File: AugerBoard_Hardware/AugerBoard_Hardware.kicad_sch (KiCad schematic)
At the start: 44 parts, among them J1 RJ45_LED_Shielded, J2 Conn_01x04_MountingPin, Q2 BSS138, Q3 BSS138, SW1 SW_SPDT, SW2 SW_Push, SW3 SW_Push, SW4 SW_Push, U1 Teensy4.1_DEV-16771, U2 OKI-78SR-5_1.5-W36H-C

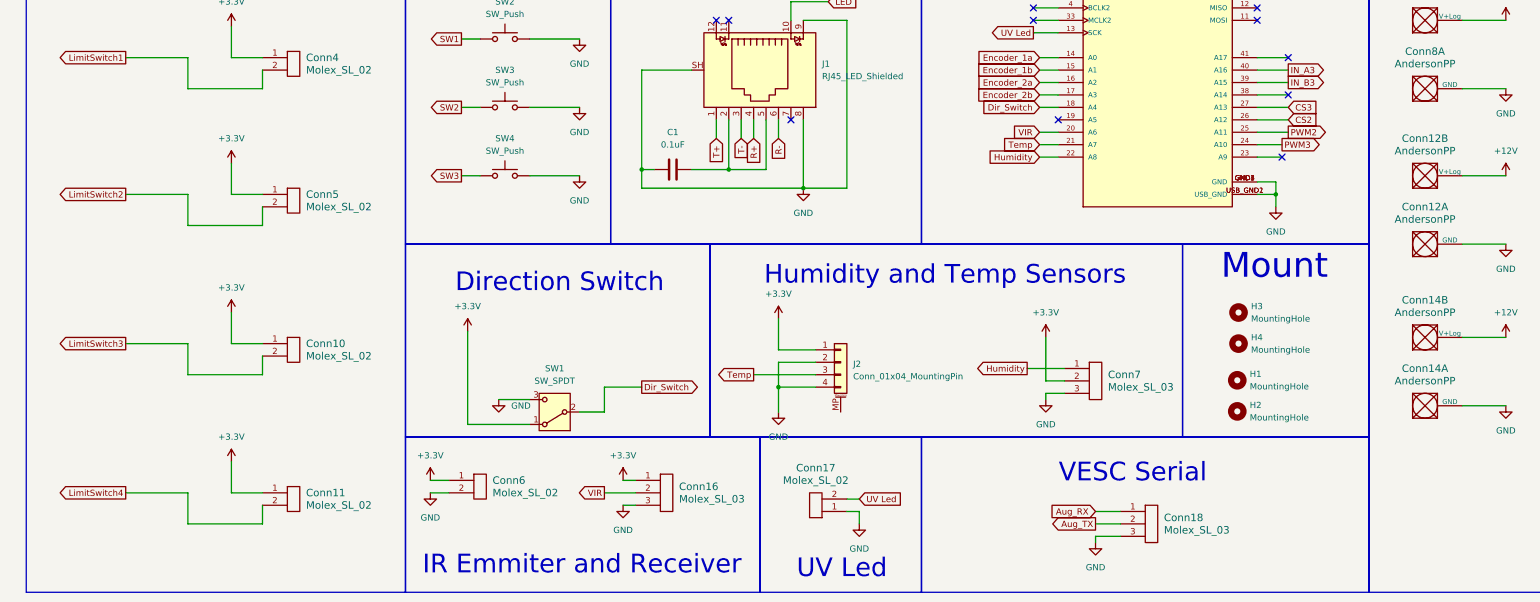
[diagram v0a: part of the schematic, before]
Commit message: Schematic probably correct, layout fucked
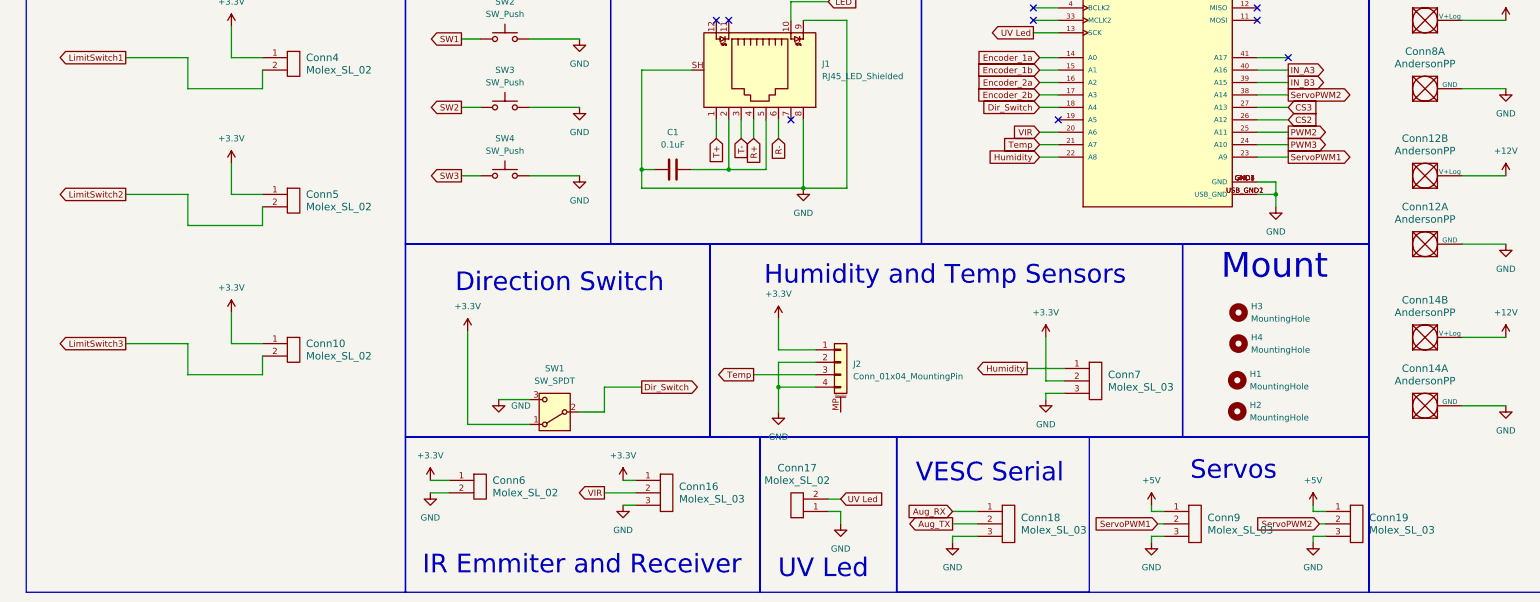
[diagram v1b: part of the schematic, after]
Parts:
- removed Conn11: Molex_SL_02, MRDT_Connectors:MOLEX_SL_02_Vertical, symbol MRDT_Connectors:Molex_SL_02
- added Conn19, Conn9: Molex_SL_03, MRDT_Connectors:MOLEX_SL_03_Vertical, symbol MRDT_Connectors:Molex_SL_03
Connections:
- net +5V: now also Conn19.1, Conn9.1
- net GND: now also Conn19.3, Conn9.3
- net ServoPWM1: now reaches U1.23 (A9)
- net ServoPWM1: now also Conn9.2
- net ServoPWM2: now reaches U1.38 (A14)
- net ServoPWM2: now also Conn19.2
- no-connect marks 25 -> 23
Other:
- note added: "Servos"
- moved on the sheet: Conn17, Conn18
